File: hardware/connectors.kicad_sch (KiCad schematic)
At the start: 9 parts, among them J1 Signals, J2 Diagnostics, J3 Power & CAN

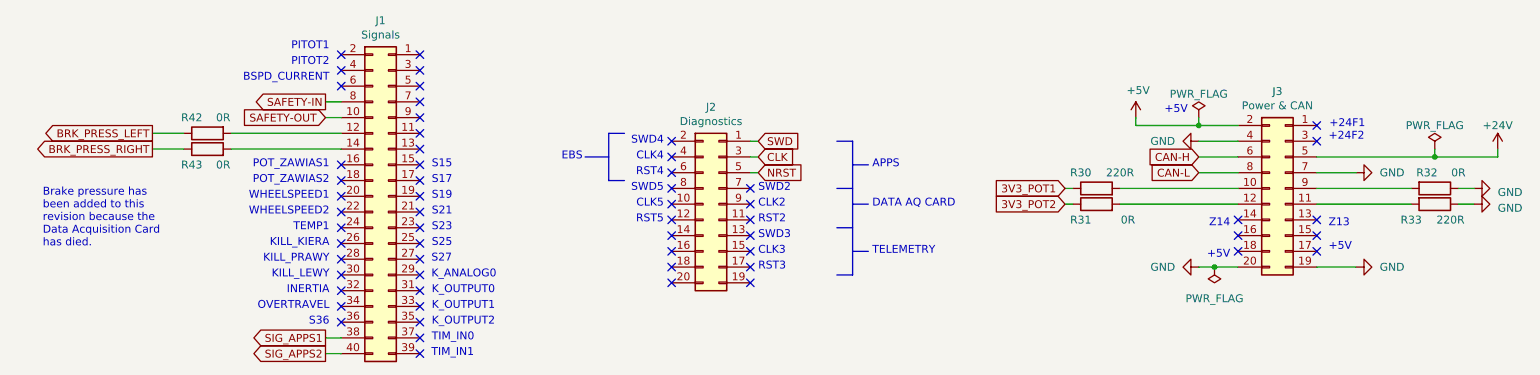
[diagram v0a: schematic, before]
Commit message: Refactor
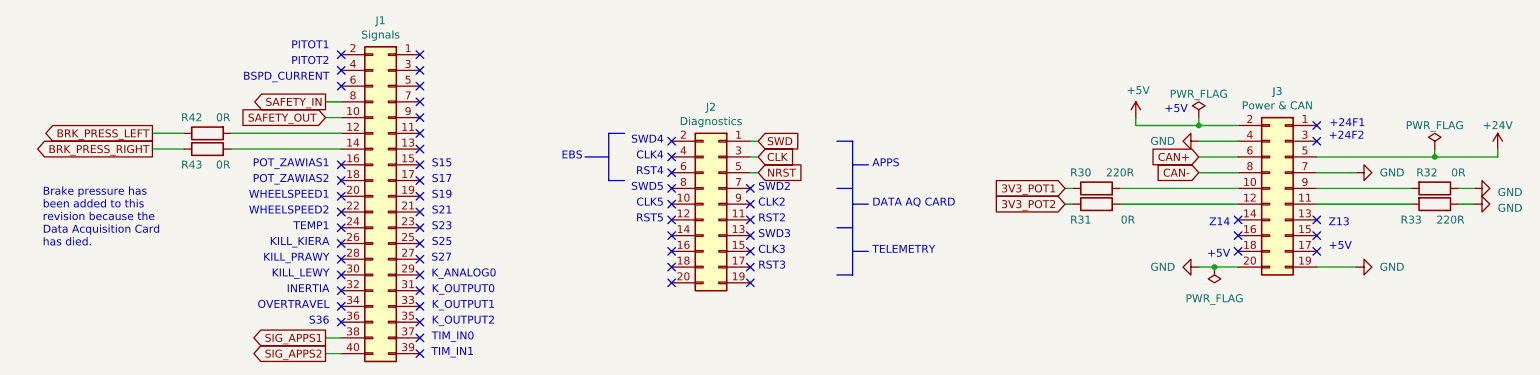
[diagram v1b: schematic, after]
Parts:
- J1: symbol conn_02x20_odd_even:Conn_02x20_Odd_Even -> Connector_Generic:Conn_02x20_Odd_Even
- J2, J3: symbol conn_02x10_odd_even:Conn_02x10_Odd_Even -> Connector_Generic:Conn_02x10_Odd_Even
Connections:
- net CAN-H renamed CAN+
- net CAN-L renamed CAN-
- net SAFETY-IN renamed SAFETY_IN
- net SAFETY-OUT renamed SAFETY_OUT
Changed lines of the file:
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@@
     (effects (font (size 1.27 1.27)) (justify left bottom))
   )
-  (global_label "SAFETY-OUT" (shape input) (at 72.39 87.63 180) (fields_autoplaced)
-    (effects (font (size 1.27 1.27)) (justify right))
-    (property "Intersheetrefs" "${INTERSHEET_REFS}" (at 58.2729 87.5506 0)
+  (global_label "SAFETY_OUT" (shape input) (at 72.39 87.63 180) (fields_autoplaced)
+    (effects (font (size 1.27 1.27)) (justify right))
+    (property "Intersheetrefs" "${INTERSHEET_REFS}" (at 58.9503 87.63 0)
       (effects (font (size 1.27 1.27)) (justify right) hide)
     )
@@
     )
   )
-  (global_label "SAFETY-IN" (shape output) (at 72.39 85.09 180) (fields_autoplaced)
-    (effects (font (size 1.27 1.27)) (justify right))
-    (property "Intersheetrefs" "${INTERSHEET_REFS}" (at 60.0388 85.09 0)
-      (effects (font (size 1.27 1.27)) (justify right) hide)
-    )
-  )
-  (global_label "CAN-L" (shape input) (at 213.36 96.52 180) (fields_autoplaced)
-    (effects (font (size 1.27 1.27)) (justify right))
-    (property "Intersheetrefs" "${INTERSHEET_REFS}" (at 204.7463 96.4406 0)
+  (global_label "SAFETY_IN" (shape output) (at 72.39 85.09 180) (fields_autoplaced)
+    (effects (font (size 1.27 1.27)) (justify right))
+    (property "Intersheetrefs" "${INTERSHEET_REFS}" (at 60.6436 85.09 0)
+      (effects (font (size 1.27 1.27)) (justify right) hide)
+    )
+  )
+  (global_label "CAN-" (shape input) (at 213.36 96.52 180) (fields_autoplaced)
+    (effects (font (size 1.27 1.27)) (justify right))
+    (property "Intersheetrefs" "${INTERSHEET_REFS}" (at 205.8469 96.52 0)
       (effects (font (size 1.27 1.27)) (justify right) hide)
     )
@@
     )
   )
-  (global_label "CAN-H" (shape input) (at 213.36 93.98 180) (fields_autoplaced)
-    (effects (font (size 1.27 1.27)) (justify right))
-    (property "Intersheetrefs" "${INTERSHEET_REFS}" (at 204.4439 93.9006 0)
+  (global_label "CAN+" (shape input) (at 213.36 93.98 180) (fields_autoplaced)
+    (effects (font (size 1.27 1.27)) (justify right))
+    (property "Intersheetrefs" "${INTERSHEET_REFS}" (at 205.8469 93.98 0)
       (effects (font (size 1.27 1.27)) (justify right) hide)
     )
@@
     (pin "2")
     (instances
-      (project "APPS"
+      (project "apps"
         (path "/fc4ad874-c922-4070-89f9-7262080469d8/00000000-0000-0000-0000-00006077b773"
           (reference "R33") (unit 1)
@@
     (pin "2")
     (instances
-      (project "APPS"
+      (project "apps"
         (path "/fc4ad874-c922-4070-89f9-7262080469d8/00000000-0000-0000-0000-00006077b773"
           (reference "R43") (unit 1)
@@
     (pin "1")
     (instances
-      (project "APPS"
+      (project "apps"
         (path "/fc4ad874-c922-4070-89f9-7262080469d8/00000000-0000-0000-0000-00006077b773"
           (reference "#PWR048") (unit 1)
@@
     (pin "1")
     (instances
-      (project "APPS"
+      (project "apps"
         (path "/fc4ad874-c922-4070-89f9-7262080469d8/00000000-0000-0000-0000-00006077b773"
           (reference "#PWR047") (unit 1)
@@
     (pin "2")
     (instances
-      (project "APPS"
+      (project "apps"
         (path "/fc4ad874-c922-4070-89f9-7262080469d8/00000000-0000-0000-0000-00006077b773"
           (reference "R42") (unit 1)
@@
     (pin "1")
     (instances
-      (project "APPS"
+      (project "apps"
         (path "/fc4ad874-c922-4070-89f9-7262080469d8/00000000-0000-0000-0000-00006077b773"
           (reference "#PWR045") (unit 1)
@@
     )
   )
-  (symbol (lib_id "conn_02x10_odd_even:Conn_02x10_Odd_Even") (at 133.35 101.6 0) (unit 1)
+  (symbol (lib_id "Connector_Generic:Conn_02x10_Odd_Even") (at 135.89 101.6 0) (mirror y) (unit 1)
     (in_bom yes) (on_board yes) (dnp no)
     (property "Reference" "J2" (at 134.62 85.9282 0)
@@
       (effects (font (size 1.27 1.27)))
     )
-    (property "Footprint" "Connector_PinSocket_2.54mm:PinSocket_2x10_P2.54mm_Vertical" (at 133.35 101.6 0)
-      (effects (font (size 1.27 1.27)) hide)
-    )
-    (property "Datasheet" "~" (at 133.35 101.6 0)
+    (property "Footprint" "Connector_PinSocket_2.54mm:PinSocket_2x10_P2.54mm_Vertical" (at 135.89 101.6 0)
+      (effects (font (size 1.27 1.27)) hide)
+    )
+    (property "Datasheet" "~" (at 135.89 101.6 0)
       (effects (font (size 1.27 1.27)) hide)
     )
@@
     (pin "9")
     (instances
-      (project "APPS"
+      (project "apps"
         (path "/fc4ad874-c922-4070-89f9-7262080469d8/00000000-0000-0000-0000-00006077b773"
           (reference "J2") (unit 1)
@@
     (pin "1")
     (instances
-      (project "APPS"
+      (project "apps"
         (path "/fc4ad874-c922-4070-89f9-7262080469d8/00000000-0000-0000-0000-00006077b773"
           (reference "#PWR043") (unit 1)
@@
     (pin "1")
     (instances
-      (project "APPS"
+      (project "apps"
         (path "/fc4ad874-c922-4070-89f9-7262080469d8/00000000-0000-0000-0000-00006077b773"
           (reference "#PWR044") (unit 1)
@@
     (pin "1")
     (instances
-      (project "APPS"
+      (project "apps"
         (path "/fc4ad874-c922-4070-89f9-7262080469d8/00000000-0000-0000-0000-00005f60f83f"
           (reference "#PWR019") (unit 1)
@@
     (pin "1")
     (instances
-      (project "APPS"
+      (project "apps"
         (path "/fc4ad874-c922-4070-89f9-7262080469d8/00000000-0000-0000-0000-00006077b773"
           (reference "#PWR046") (unit 1)
@@
     )
   )
-  (symbol (lib_id "conn_02x10_odd_even:Conn_02x10_Odd_Even") (at 224.79 99.06 0) (unit 1)
+  (symbol (lib_id "Connector_Generic:Conn_02x10_Odd_Even") (at 227.33 99.06 0) (mirror y) (unit 1)
     (in_bom yes) (on_board yes) (dnp no)
     (property "Reference" "J3" (at 226.06 83.3882 0)
@@
       (effects (font (size 1.27 1.27)))
     )
-    (property "Footprint" "Connector_PinSocket_2.54mm:PinSocket_2x10_P2.54mm_Vertical" (at 224.79 99.06 0)
-      (effects (font (size 1.27 1.27)) hide)
-    )
-    (property "Datasheet" "~" (at 224.79 99.06 0)
+    (property "Footprint" "Connector_PinSocket_2.54mm:PinSocket_2x10_P2.54mm_Vertical" (at 227.33 99.06 0)
+      (effects (font (size 1.27 1.27)) hide)
+    )
+    (property "Datasheet" "~" (at 227.33 99.06 0)
       (effects (font (size 1.27 1.27)) hide)
     )
@@
     (pin "9")
     (instances
-      (project "APPS"
+      (project "apps"
         (path "/fc4ad874-c922-4070-89f9-7262080469d8/00000000-0000-0000-0000-00006077b773"
           (reference "J3") (unit 1)
@@
     (pin "1")
     (instances
-      (project "APPS"
+      (project "apps"
         (path "/fc4ad874-c922-4070-89f9-7262080469d8/00000000-0000-0000-0000-00006077b773"
           (reference "#FLG02") (unit 1)
@@
     (pin "1")
     (instances
-      (project "APPS"
+      (project "apps"
         (path "/fc4ad874-c922-4070-89f9-7262080469d8/00000000-0000-0000-0000-00006077b773"
           (reference "#FLG04") (unit 1)
@@
     )
   )
-  (symbol (lib_id "conn_02x20_odd_even:Conn_02x20_Odd_Even") (at 80.01 100.33 0) (unit 1)
+  (symbol (lib_id "Connector_Generic:Conn_02x20_Odd_Even") (at 82.55 100.33 0) (mirror y) (unit 1)
     (in_bom yes) (on_board yes) (dnp no)
     (property "Reference" "J1" (at 81.28 71.9582 0)
@@
       (effects (font (size 1.27 1.27)))
     )
-    (property "Footprint" "Connector_PinSocket_2.54mm:PinSocket_2x20_P2.54mm_Vertical" (at 80.01 100.33 0)
-      (effects (font (size 1.27 1.27)) hide)
-    )
-    (property "Datasheet" "~" (at 80.01 100.33 0)
+    (property "Footprint" "Connector_PinSocket_2.54mm:PinSocket_2x20_P2.54mm_Vertical" (at 82.55 100.33 0)
+      (effects (font (size 1.27 1.27)) hide)
+    )
+    (property "Datasheet" "~" (at 82.55 100.33 0)
       (effects (font (size 1.27 1.27)) hide)
     )
@@
     (pin "9")
     (instances
-      (project "APPS"
+      (project "apps"
         (path "/fc4ad874-c922-4070-89f9-7262080469d8/00000000-0000-0000-0000-00006077b773"
           (reference "J1") (unit 1)
@@
     (pin "1")
     (instances
-      (project "APPS"
+      (project "apps"
         (path "/fc4ad874-c922-4070-89f9-7262080469d8/00000000-0000-0000-0000-00006077b773"
           (reference "#PWR042") (unit 1)
@@
     (pin "2")
     (instances
-      (project "APPS"
+      (project "apps"
         (path "/fc4ad874-c922-4070-89f9-7262080469d8/00000000-0000-0000-0000-00006077b773"
           (reference "R30") (unit 1)
@@
     (pin "2")
     (instances
-      (project "APPS"
+      (project "apps"
         (path "/fc4ad874-c922-4070-89f9-7262080469d8/00000000-0000-0000-0000-00006077b773"
           (reference "R32") (unit 1)
@@
     (pin "2")
     (instances
-      (project "APPS"
+      (project "apps"
         (path "/fc4ad874-c922-4070-89f9-7262080469d8/00000000-0000-0000-0000-00006077b773"
           (reference "R31") (unit 1)
@@
     (pin "1")
     (instances
-      (project "APPS"
+      (project "apps"
         (path "/fc4ad874-c922-4070-89f9-7262080469d8/00000000-0000-0000-0000-00006077b773"
           (reference "#FLG03") (unit 1)
